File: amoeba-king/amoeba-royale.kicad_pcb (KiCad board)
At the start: 2 copper layers, 19.1 x 19.1 mm, 7 parts, among them J1 Conn_01x05_Male, J2 Conn_01x05_Male, J3 Conn_01x04_Male, J4 Conn_01x05_Male

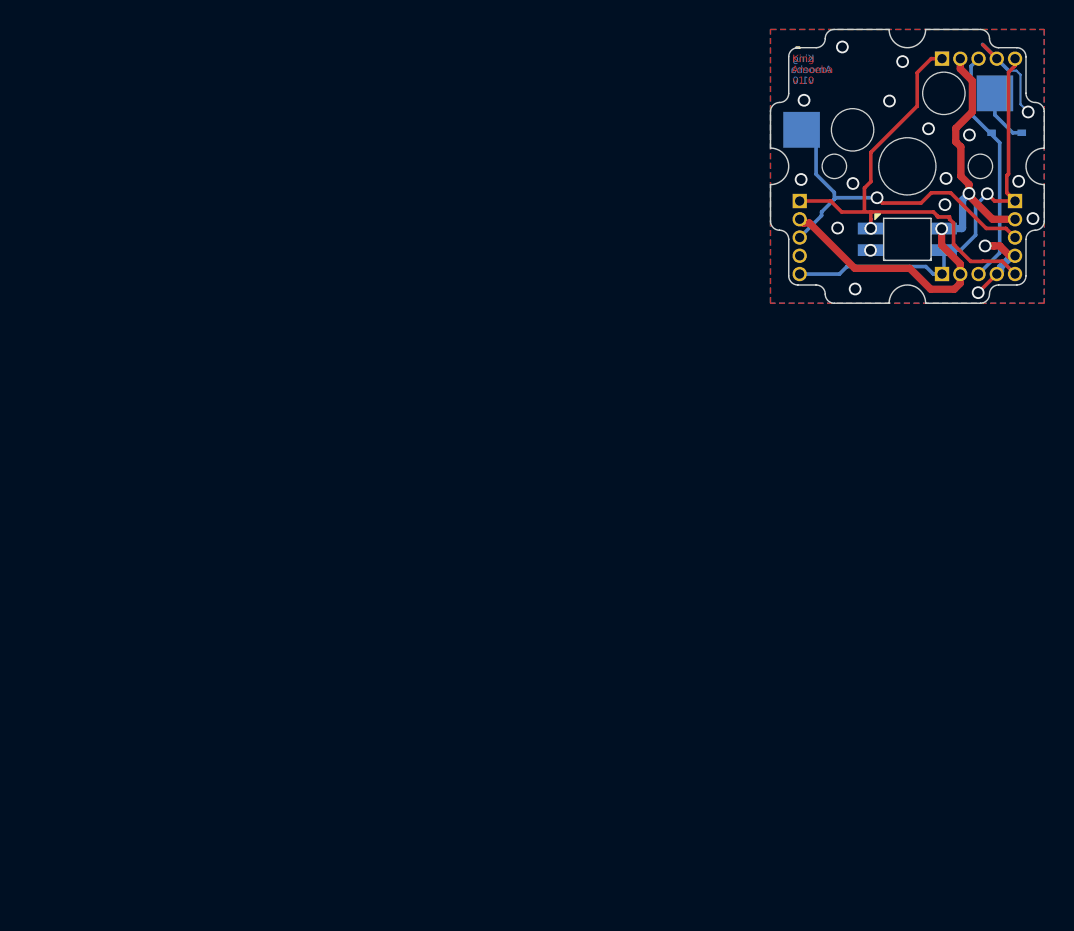
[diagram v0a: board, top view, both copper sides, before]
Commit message: Getting ready for final review, before sending for production
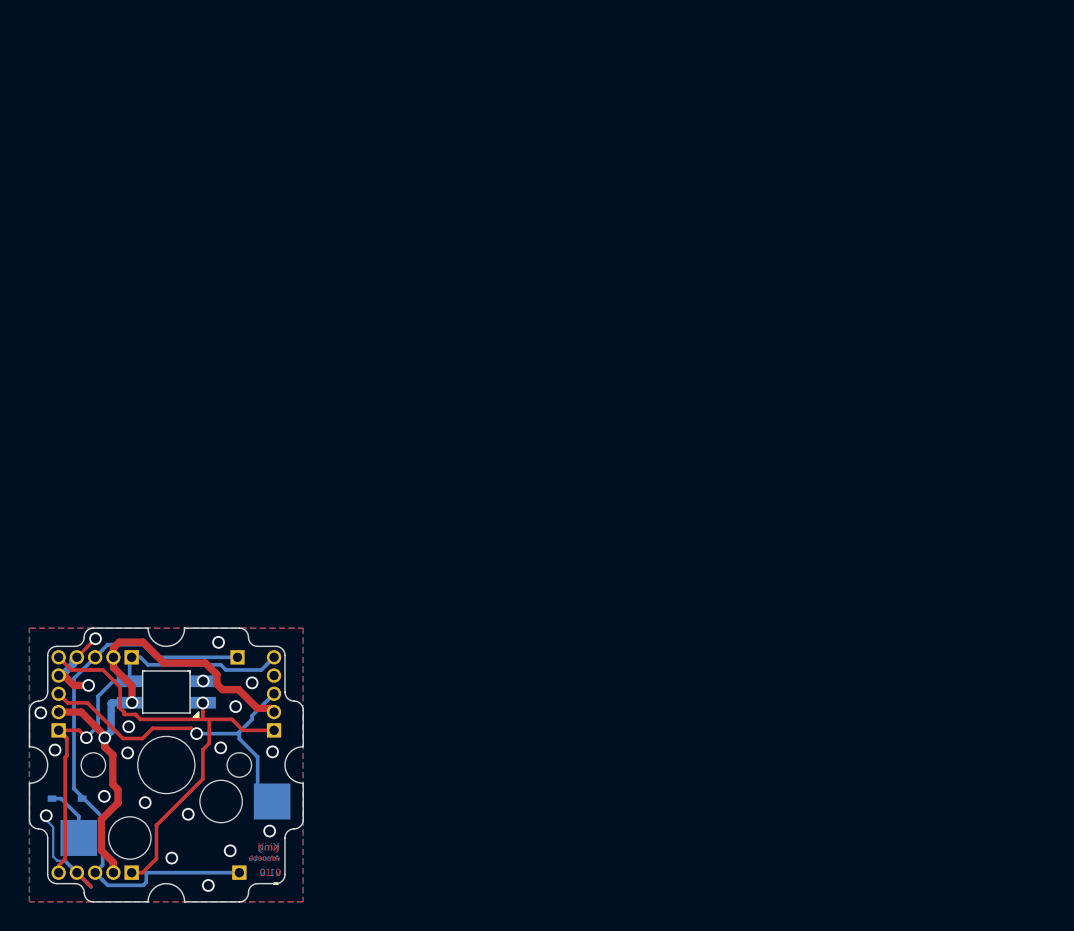
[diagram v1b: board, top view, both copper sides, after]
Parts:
- added J5: Conn_01x01_Male, amoeba-modules:Header_1x01_P1.27mm, B.Cu at (80.5, 176.1)
- added J6: Conn_01x01_Male, amoeba-modules:Header_1x01_P1.27mm, B.Cu at (80.4, 161.2)
- moved D1 80.1 mm to (68.5, 171.0), turned to 180 degrees
- moved J1 79.9 mm to (73.0, 176.1), turned to 90 degrees
- moved J2 76.1 mm to (67.9, 166.2), turned to 0 degrees
- moved S1 66.3 mm to (75.4, 168.7), turned to 0 degrees
- moved J3 62.4 mm to (73.0, 161.2), turned to 90 degrees
- moved LED1 60.4 mm to (75.4, 163.6), turned to 180 degrees
- moved J4 51.9 mm to (82.9, 166.2), turned to 0 degrees
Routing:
- net /C: track 16.6 -> 38.4 mm
- net /GND: vias 18 -> 20
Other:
- board size 19.1 x 19.1 mm -> 19 x 19.1 mm
- board text added: "C"
- board text added: "DI"
- board text added: "DO"
- board text added: "G"
- board text added: "R"
- board text added: "V"
